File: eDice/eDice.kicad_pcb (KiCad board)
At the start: 2 copper layers, 25 parts, among them Q1 PMOS, Q2 PN2222A, Q3 PN2222A, SW1 SW_Push, U1 NE555P, U10 4511, U11 SM420561N, U12 4029, U2 4029, U3 4511, U4 SM420561N

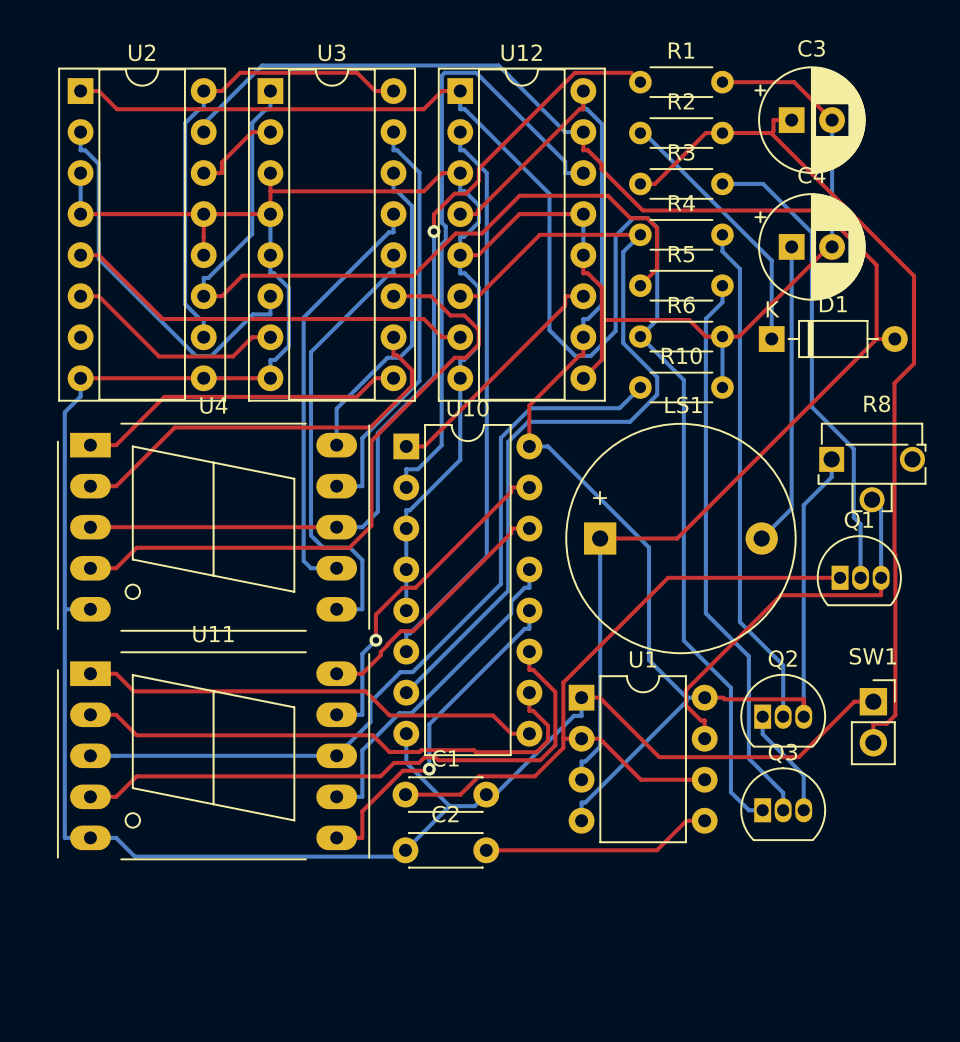
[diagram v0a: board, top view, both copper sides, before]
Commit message: updates
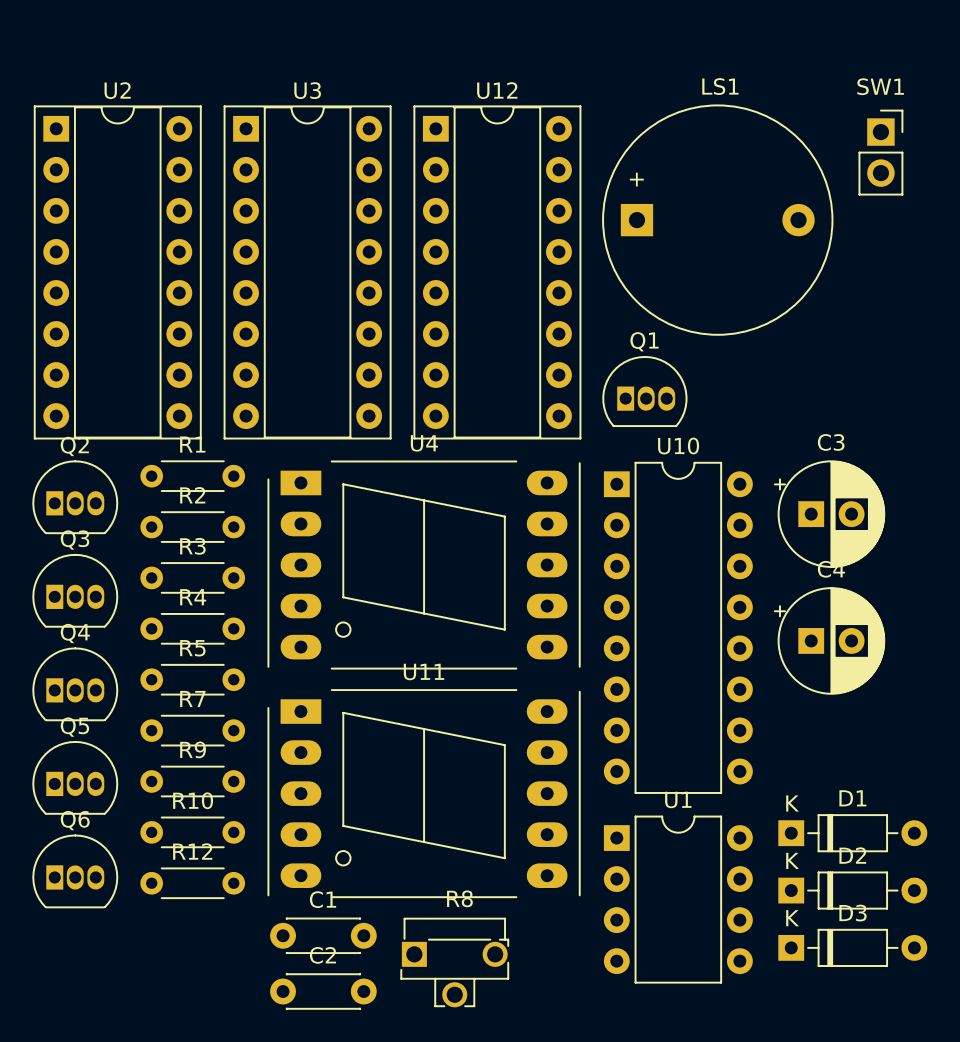
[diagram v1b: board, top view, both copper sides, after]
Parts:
- removed R6: 100k, Resistor_THT:R_Axial_DIN0204_L3.6mm_D1.6mm_P5.08mm_Horizontal
- added D2: 1N4148, Diode_THT:D_DO-35_SOD27_P7.62mm_Horizontal, F.Cu at (180.3, 123.5)
- added D3: 1N4148, Diode_THT:D_DO-35_SOD27_P7.62mm_Horizontal, F.Cu at (180.3, 127.0)
- added Q4: PN2222A, Package_TO_SOT_THT:TO-92_Inline, F.Cu at (134.8, 111.1)
- added Q5: PN2222A, Package_TO_SOT_THT:TO-92_Inline, F.Cu at (134.8, 116.8)
- added Q6: PN2222A, Package_TO_SOT_THT:TO-92_Inline, F.Cu at (134.8, 122.6)
- added R12: 10k, Resistor_THT:R_Axial_DIN0204_L3.6mm_D1.6mm_P5.08mm_Horizontal, F.Cu at (140.8, 123.0)
- added R7: 10k, Resistor_THT:R_Axial_DIN0204_L3.6mm_D1.6mm_P5.08mm_Horizontal, F.Cu at (140.8, 113.5)
- added R9: 10k, Resistor_THT:R_Axial_DIN0204_L3.6mm_D1.6mm_P5.08mm_Horizontal, F.Cu at (140.8, 116.7)
- moved Q2 45.8 mm to (134.8, 99.5)
- moved Q3 45.8 mm to (134.8, 105.3)
- moved R10 40.9 mm to (140.8, 119.8)
- moved R8 40.1 mm to (157.0, 127.4)
- moved R1 38.9 mm to (140.8, 97.8)
- moved R2 38.9 mm to (140.8, 101.0)
- moved R3 38.9 mm to (140.8, 104.1)
- moved R4 38.9 mm to (140.8, 107.2)
- moved R5 38.9 mm to (140.8, 110.4)
- moved SW1 35.3 mm to (185.9, 76.5)
- moved D1 30.6 mm to (180.3, 119.9)
- moved C3 24.4 mm to (181.6, 100.2)
- moved C4 24.4 mm to (181.6, 108.0)
- moved LS1 19.8 mm to (170.8, 82.0)
- moved Q1 17.3 mm to (170.1, 93.0)
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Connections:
- Q2 pad 1: Net-(Q2-E) -> GND
- Q2 pad 3: vcc -> Net-(Q2-C)
- Q3 pad 3: Net-(Q2-E) -> Net-(Q3-C)
- R1 pad 2: GND -> Net-(Q2-C)
- R4 pad 1: Net-(U10-DA) -> Net-(Q4-B)
- R4 pad 2: Net-(Q2-B) -> Net-(Q3-C)
- U10 pad 3: GND -> vcc
- U10 pad 4: GND -> vcc
- U10 pad 7: Net-(U10-DA) -> Net-(Q3-C)
- U12 pad 6: Net-(U10-DA) -> Net-(Q3-C)
- U2 pad 10: Net-(U2-U/D) -> vcc
- U2 pad 16: Net-(U2-U/D) -> vcc
- U3 pad 16: Net-(U2-U/D) -> vcc
- U3 pad 3: GND -> vcc
- U3 pad 4: GND -> vcc
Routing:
- net GND: track 235.8 -> 0.00 mm
- net PE: track 96.4 -> 0.00 mm
- net clck: track 93.1 -> 0.00 mm
- net vcc: track 92.1 -> 0.00 mm
- net Net-(R1-Pad1): track 55.1 -> 0.00 mm, vias 1 -> 0
- net Net-(C3-Pad1): track 54.4 -> 0.00 mm
- net Net-(U10-DA): track 52.5 -> 0.00 mm
- net Net-(U2-Q2): track 50.2 -> 0.00 mm
- net Net-(R10-Pad1): track 49.5 -> 0.00 mm
- net Net-(Q1-D): track 44.6 -> 0.00 mm
- net Net-(U3-Qc): track 39.9 -> 0.00 mm
- net Net-(U10-DC): track 38.8 -> 0.00 mm
- net Net-(U10-Qc): track 36.8 -> 0.00 mm
- net Net-(Q6-C): track 35.2 -> 0.00 mm
- net Net-(Q3-B): track 34.9 -> 0.00 mm
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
